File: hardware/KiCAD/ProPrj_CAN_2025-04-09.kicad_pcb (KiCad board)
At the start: 2 copper layers, 66 x 50 mm, 27 parts, among them J1 BOOT, J2 PROG, J3 KF2510-4, U1 LM2575-5.0BT, U2 MCP2515-I, U3 AMS1117-3.3, U4 TJA1050DRG, U5 ESP-12F, Y1 Crystal

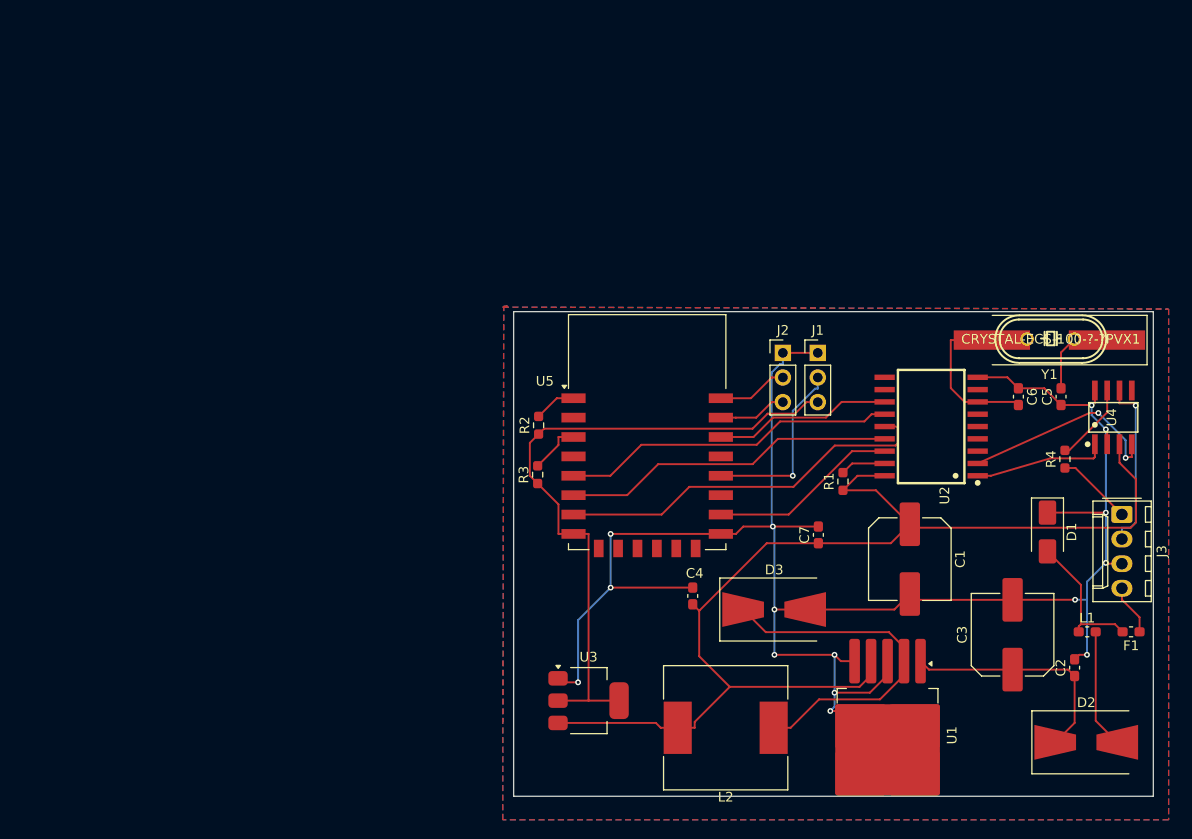
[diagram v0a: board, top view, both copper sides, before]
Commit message: Rouring
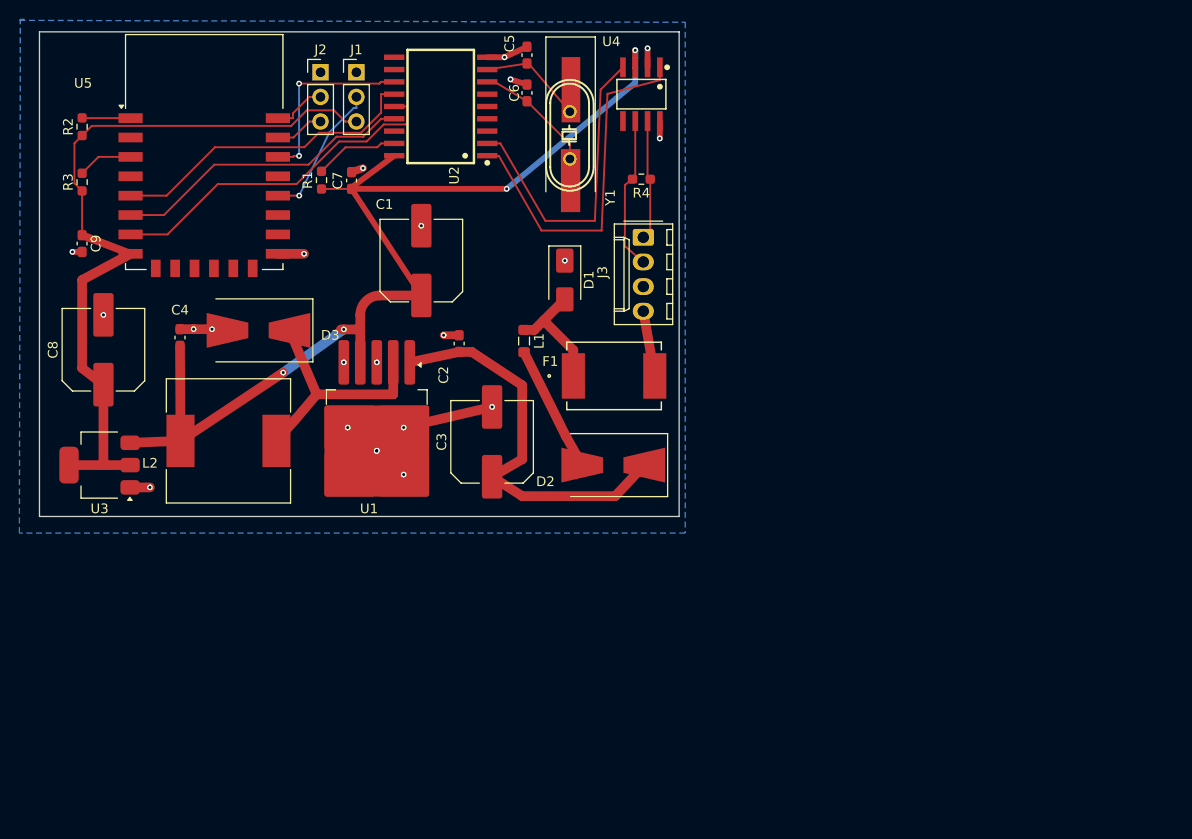
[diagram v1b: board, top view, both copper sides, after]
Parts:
- removed CRYSTAL-ECS-100-?-?PVX1: 8MHz, ProPrj_CAN_2025-04-09:HC-49US_L11.5-W4.5-P4.88
- added C8: 470 uF, Capacitor_SMD:C_Elec_8x10.2, F.Cu at (106.6, 82.8)
- added C9: 100 nF, Capacitor_SMD:C_0603_1608Metric_Pad1.08x0.95mm_HandSolder, F.Cu at (104.4, 71.8)
- F1: footprint Inductor_SMD:L_0603_1608Metric_Pad1.05x0.95mm_HandSolder -> Library:FUSE_MF-SM185_BRN
- L1: value BLM18PG121SN1D -> BLM21PG300SN1D; footprint Inductor_SMD:L_0603_1608Metric_Pad1.05x0.95mm_HandSolder -> Inductor_SMD:L_0805_2012Metric_Pad1.05x1.20mm_HandSolder
- Y1: value Crystal -> 8 - 16 MHz; footprint Crystal:Crystal_SMD_HC49-SD_HandSoldering -> Library:Crystal_SMD_HC49-SD_HandSoldering
- moved C2 71.8 mm to (143.3, 82.2)
- moved C5 65.4 mm to (150.3, 52.4), turned to -90 degrees
- moved L1 65.4 mm to (150.0, 81.9), turned to -90 degrees
- moved R1 62.1 mm to (129.1, 65.3)
- moved U1 61.1 mm to (134.8, 91.8)
- moved D3 60.5 mm to (122.6, 80.8), turned to 180 degrees
- moved C7 60.5 mm to (132.2, 65.3)
- moved U2 60.4 mm to (141.4, 57.7)
- moved C6 59.6 mm to (150.3, 56.3)
- moved F1 59.5 mm to (159.3, 85.5), turned to 0 degrees
- moved C4 59.2 mm to (114.5, 81.5)
- moved L2 59.2 mm to (119.5, 92.2)
- moved C1 59.1 mm to (139.4, 73.6), turned to 90 degrees
- moved U4 59.0 mm to (162.1, 56.4), turned to -90 degrees
- moved C3 57.3 mm to (146.7, 92.3)
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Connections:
- F1 pad 1: +12V -> Net-(D1-A2)
- F1 pad 2: Net-(D1-A2) -> +12V
- R4 pad 2: Net-(U4-CANH) -> Net-(J3-Pin_2)
- U4 pad 7: Net-(U4-CANH) -> Net-(J3-Pin_1)
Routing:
- net GND: track 212.4 -> 50.8 mm, vias 15 -> 22
- net Net-(U2-TXCAN): track 13.7 -> 37.3 mm
- net Net-(U2-~CS~): track 19.6 -> 0.00 mm
- net Net-(D2-K): track 24.2 -> 41.6 mm
- net Net-(D3-K): track 36.8 -> 24.7 mm
- net Net-(U2-RXCAN): track 21.4 -> 32.5 mm, vias 2 -> 0
- net +3.3V: track 68.7 -> 78.3 mm
- net Net-(U4-CANH): track 8.24 -> 0.00 mm
- net VCC: track 118.7 -> 113.1 mm, vias 0 -> 4
- net Net-(U2-OSC2): track 20.6 -> 15.9 mm
- net Net-(J3-Pin_1): track 7.86 -> 12.4 mm
- net Net-(J1-Pin_2): track 18.8 -> 14.7 mm
- net Net-(U2-~RESET~): track 4.69 -> 8.69 mm
- net Net-(U2-SI): track 39.6 -> 36.4 mm
- net Net-(U2-SO): track 34.5 -> 31.3 mm
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- removed copper zone on F.Cu, net GND
